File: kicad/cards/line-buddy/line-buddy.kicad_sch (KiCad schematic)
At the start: 18 parts, among them J1 Conn_01x06_Pin, J2 Conn_01x06_Pin, J4 Conn_01x05, U1 THVD1450DR, U2 STM32C011F4Px

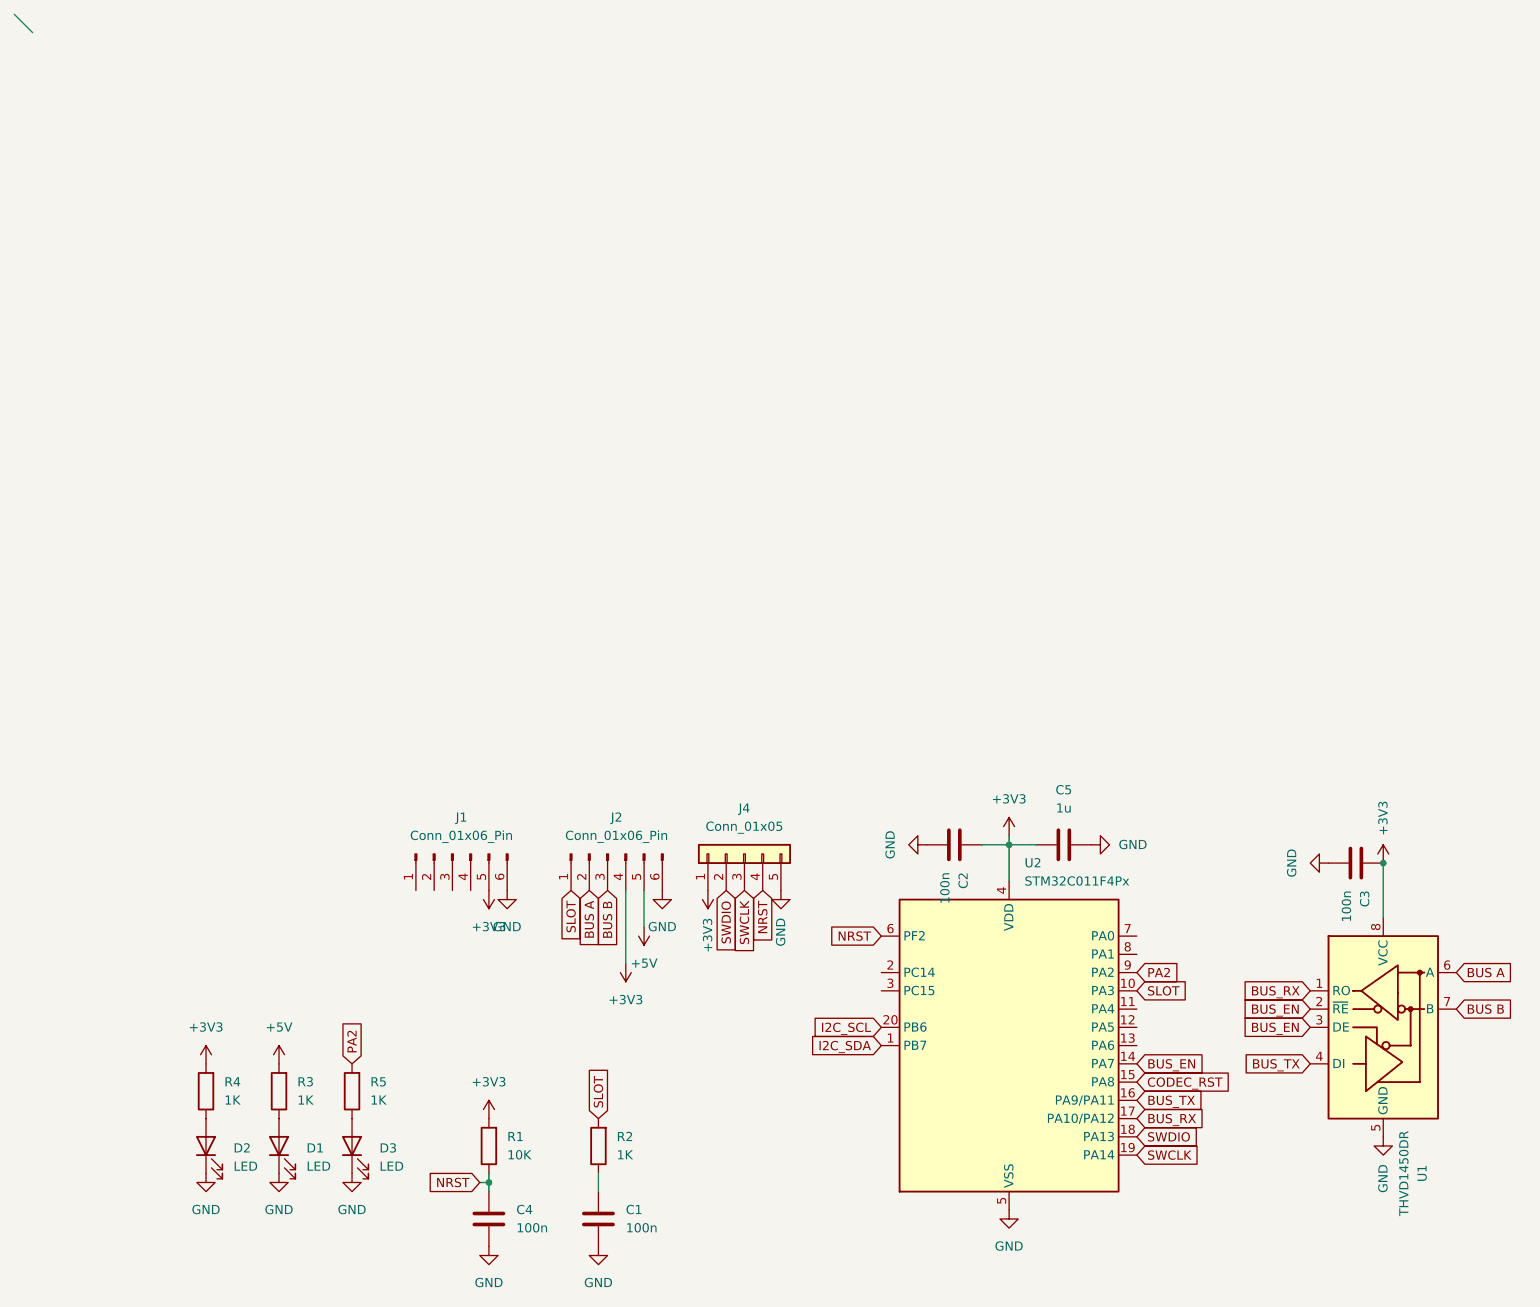
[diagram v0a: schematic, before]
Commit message: Add new line buddy WIP
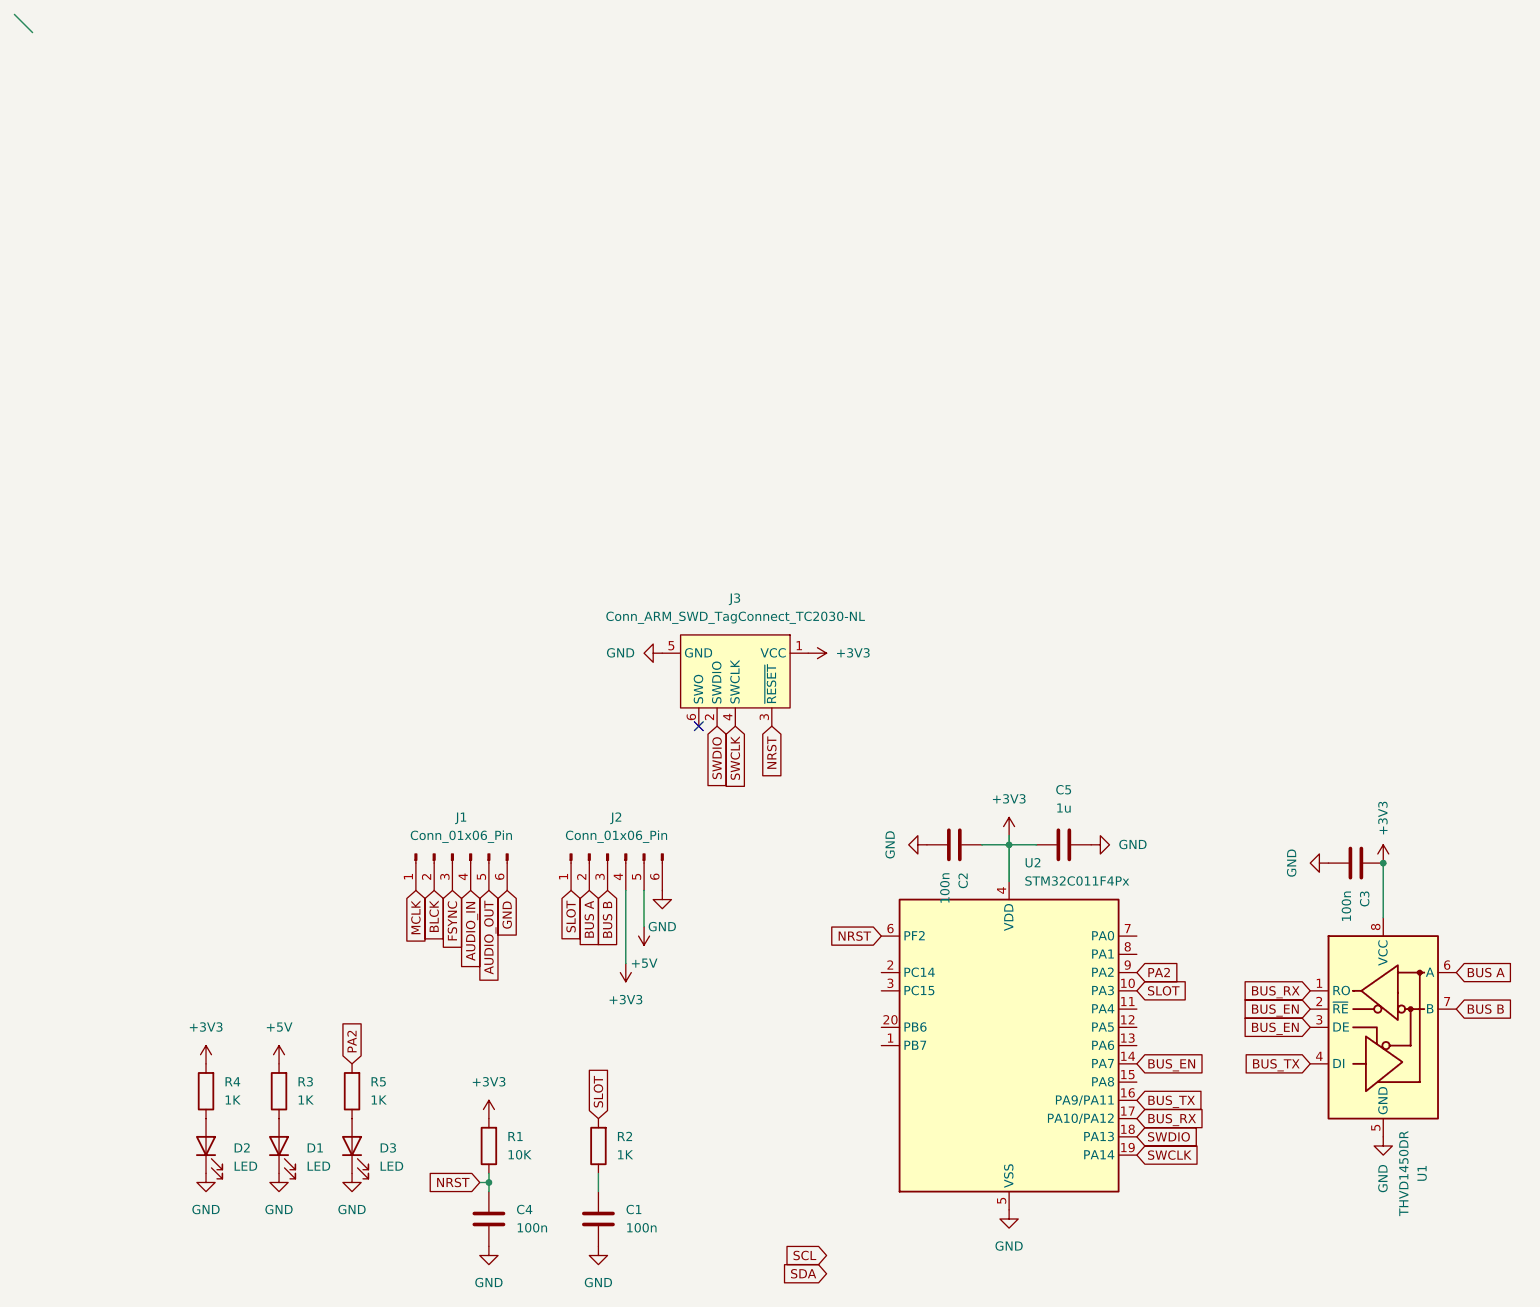
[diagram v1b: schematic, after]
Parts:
- removed J4: Conn_01x05, Connector_PinHeader_1.27mm:PinHeader_1x05_P1.27mm_Vertical, symbol Connector_Generic:Conn_01x05
- added J3: Conn_ARM_SWD_TagConnect_TC2030-NL, Connector:Tag-Connect_TC2030-IDC-NL_2x03_P1.27mm_Vertical, symbol Connector:Conn_ARM_SWD_TagConnect_TC2030-NL
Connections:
- net +3V3: now also J3.1 (VCC); no longer J1.5 (Pin_5)
- net GND: now also J3.5 (GND)
- net NRST: now also J3.3 (~{RESET})
- net SWCLK: now also J3.4 (SWCLK)
- net SWDIO: now also J3.2 (SWDIO)
- net MCLK: now reaches J1.1 (Pin_1)
- net BLCK: now reaches J1.2 (Pin_2)
- net FSYNC: now reaches J1.3 (Pin_3)
- net AUDIO_IN: now reaches J1.4 (Pin_4)
- net CODEC_RST: no longer names the net of U2.15 (PA8)
- net I2C_SCL: no longer names the net of U2.20 (PB6)
- net I2C_SDA: no longer names the net of U2.1 (PB7)
- new net AUDIO_OUT: J1.5 (Pin_5)
- no-connect marks 0 -> 1

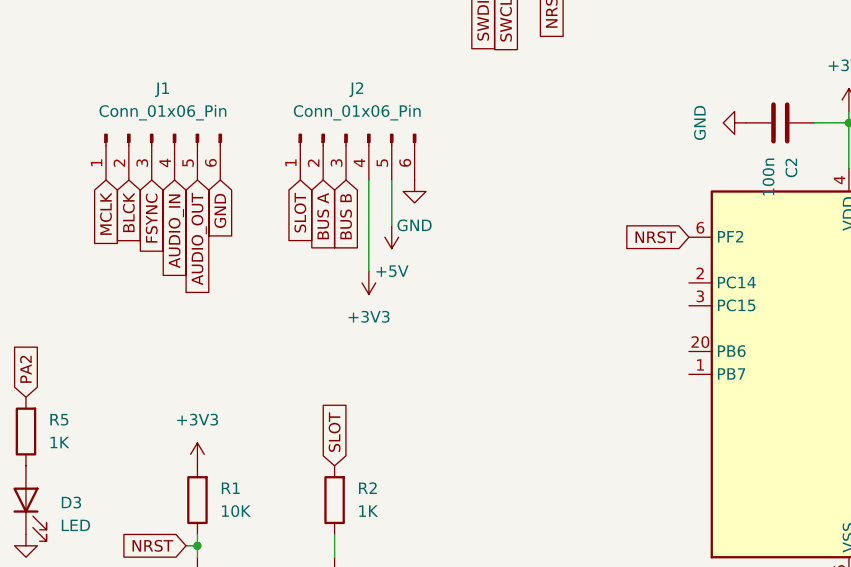
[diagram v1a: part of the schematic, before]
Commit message: Finish Line Buddy
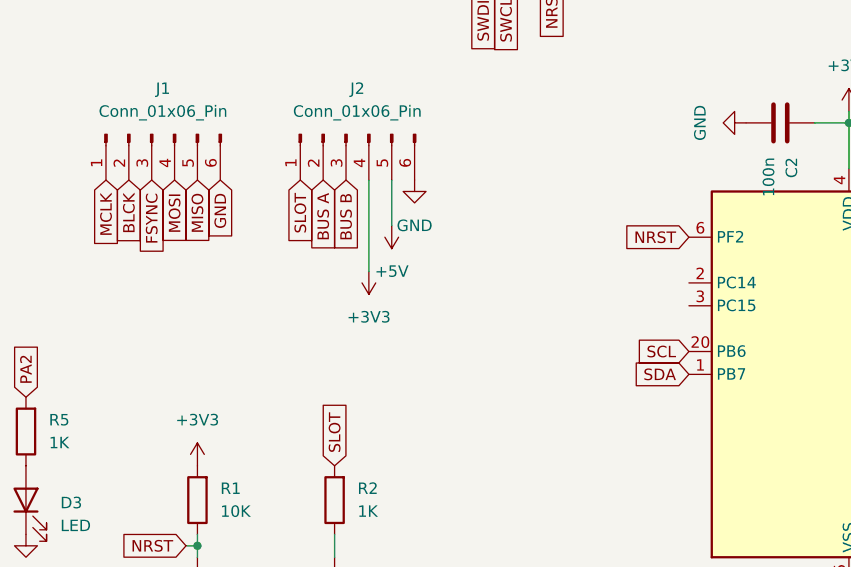
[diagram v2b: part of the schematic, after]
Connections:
- net SCL: now also U2.20 (PB6)
- net SDA: now also U2.1 (PB7)
- net AUDIO_IN renamed MOSI
- net AUDIO_OUT renamed MISO
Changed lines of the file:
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@@
 		)
 	)
-	(global_label "AUDIO_IN"
+	(global_label "MOSI"
 		(shape input)
 		(at 82.55 82.55 270)
@@
 		)
 		(property "Intersheetrefs" "${INTERSHEET_REFS}"
-			(at 82.55 94.0625 90)
+			(at 82.55 90.1314 90)
 			(hide yes)
 			(show_name no)
@@
 		)
 	)
+	(global_label "SCL"
+		(shape input)
+		(at 139.7 101.6 180)
+		(fields_autoplaced yes)
+		(effects
+			(font
+				(size 1.27 1.27)
+			)
+			(justify right)
+		)
+		(property "Intersheetrefs" "${INTERSHEET_REFS}"
+			(at 133.2072 101.6 0)
+			(hide yes)
+			(show_name no)
+			(do_not_autoplace no)
+			(effects
+				(font
+					(size 1.27 1.27)
+				)
+				(justify right)
+			)
+		)
+	)
 	(global_label "BUS_RX"
 		(shape input)
@@
 		)
 	)
+	(global_label "SDA"
+		(shape input)
+		(at 139.7 104.14 180)
+		(fields_autoplaced yes)
+		(effects
+			(font
+				(size 1.27 1.27)
+			)
+			(justify right)
+		)
+		(property "Intersheetrefs" "${INTERSHEET_REFS}"
+			(at 133.1467 104.14 0)
+			(hide yes)
+			(show_name no)
+			(do_not_autoplace no)
+			(effects
+				(font
+					(size 1.27 1.27)
+				)
+				(justify right)
+			)
+		)
+	)
 	(global_label "PA2"
 		(shape input)
@@
 		)
 	)
-	(global_label "AUDIO_OUT"
+	(global_label "MISO"
 		(shape input)
 		(at 85.09 82.55 270)
@@
 		)
 		(property "Intersheetrefs" "${INTERSHEET_REFS}"
-			(at 85.09 95.7558 90)
-			(hide yes)
-			(show_name no)
+			(at 85.09 90.1314 90)
+			(hide yes)
+			(show_name no)
